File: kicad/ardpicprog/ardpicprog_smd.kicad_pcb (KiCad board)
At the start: 2 copper layers, 69.2 x 53.9 mm, 37 parts, among them P1 CONN_01X06, P2 CONN_01X02, Q1 BC548, SW1 SW_PUSH, U1 PIC16F627, U2 MC34063, U3 LM78L12ACZ

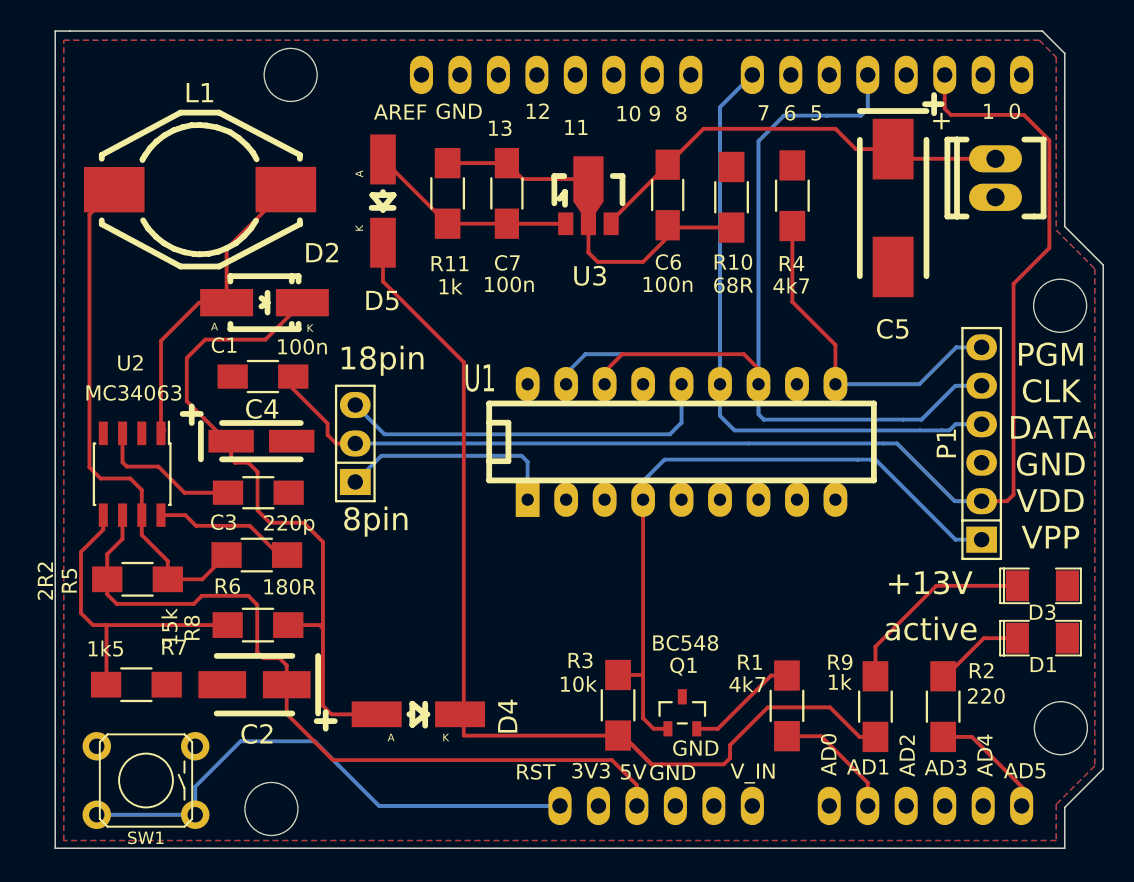
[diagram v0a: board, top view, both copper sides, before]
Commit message: to fcking much changes to commit it separatly, lets go with everything in one commit, git will love me for sure :D
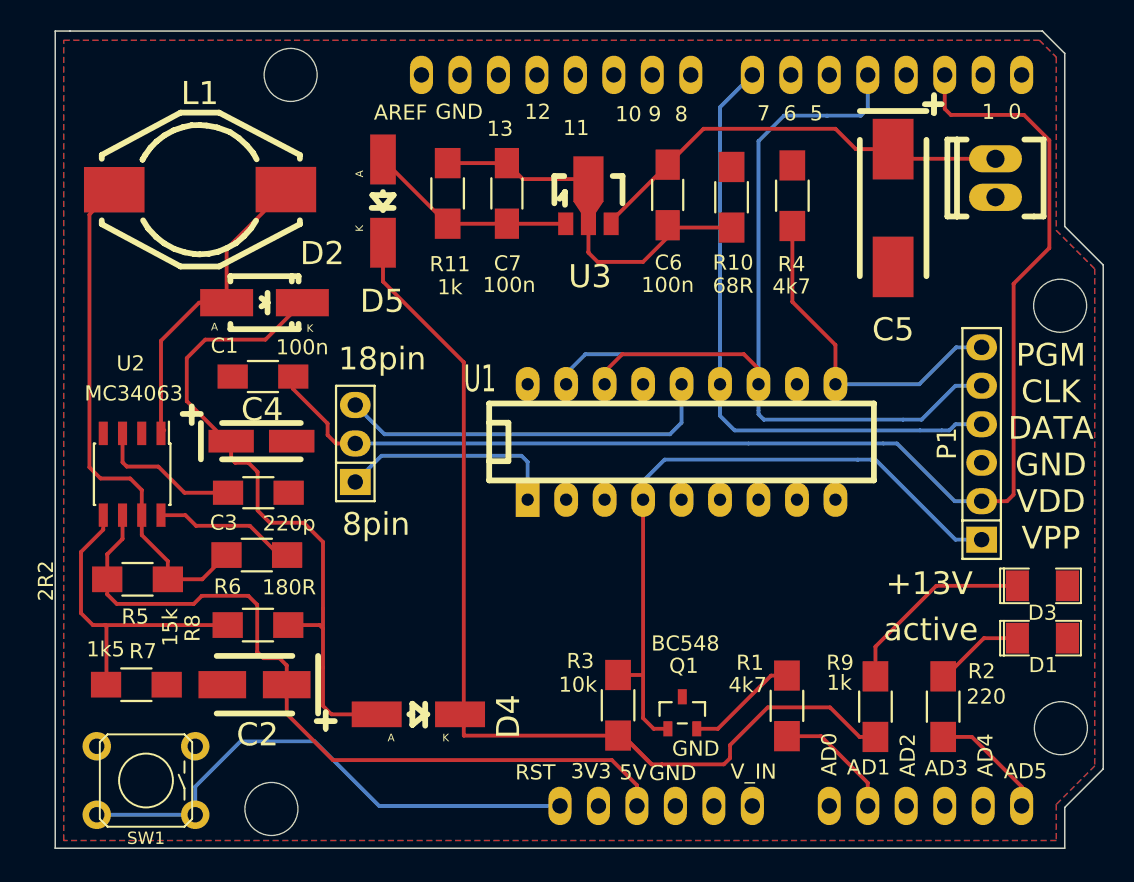
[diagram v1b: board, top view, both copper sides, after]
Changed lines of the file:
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@@
-(kicad_pcb (version 20160815) (host pcbnew 4.1.0-alpha+201608211231+7083~46~ubuntu16.04.1-product)
+(kicad_pcb (version 20171130) (host pcbnew 5.0.0-rc2-dev-unknown-ce1bd4c~62~ubuntu16.04.1)
   (general
-    (links 74)
-    (no_connects 1)
-    (area 129.286799 76.099199 198.576401 130.148801)
     (thickness 1.6)
     (drawings 34)
@@
     (pad_to_mask_clearance 0)
     (aux_axis_origin 0 0)
-    (visible_elements FFFFFF7F)
+    (visible_elements FFFDFF7F)
     (pcbplotparams
-      (layerselection 0x00030_80000001)
+      (layerselection 0x010fc_ffffffff)
       (usegerberextensions false)
+      (usegerberattributes false)
+      (usegerberadvancedattributes false)
+      (creategerberjobfile false)
       (excludeedgelayer true)
       (linewidth 0.100000)
@@
       (drillshape 0)
       (scaleselection 1)
-      (outputdirectory ""))
+      (outputdirectory /home/nail/src/hw/kicad/ardpicprog/prod/))
   )
   (net 0 "")
@@
     (uvia_dia 0.508)
     (uvia_drill 0.127)
-    (diff_pair_gap 0.25)
-    (diff_pair_width 0.2)
     (add_net 13V)
     (add_net 5V)
@@
     (attr smd)
     (fp_text reference C4 (at 0.0508 -2.0828 180) (layer F.SilkS)
-      (effects (font (thickness 0.3048)))
+      (effects (font (size 1.524 1.524) (thickness 0.3048)))
     )
     (fp_text value 10m/16V (at -0.09906 3.0988) (layer F.SilkS) hide
-      (effects (font (thickness 0.3048)))
+      (effects (font (size 1.524 1.524) (thickness 0.3048)))
     )
     (fp_text user + (at -4.59994 -1.80086) (layer F.SilkS)
-      (effects (font (thickness 0.3048)))
+      (effects (font (size 1.524 1.524) (thickness 0.3048)))
     )
     (fp_line (start -2.60096 1.19888) (end 2.60096 1.19888) (layer F.SilkS) (width 0.381))
@@
     (attr smd)
     (fp_text reference C5 (at 8.0264 0) (layer F.SilkS)
-      (effects (font (thickness 0.3048)))
+      (effects (font (size 1.524 1.524) (thickness 0.3048)))
     )
     (fp_text value 33m/35V (at -0.09906 3.59918 270) (layer F.SilkS) hide
-      (effects (font (thickness 0.3048)))
+      (effects (font (size 1.524 1.524) (thickness 0.3048)))
     )
     (fp_line (start -6.40334 -2.19964) (end -6.40334 2.19964) (layer F.SilkS) (width 0.381))
     (fp_line (start -4.50088 2.19964) (end 4.50088 2.19964) (layer F.SilkS) (width 0.381))
     (fp_line (start 4.50088 -2.19964) (end -4.50088 -2.19964) (layer F.SilkS) (width 0.381))
-    (fp_text user + (at -5.7404 -3.1496 270) (layer F.SilkS)
-      (effects (font (thickness 0.3048)))
+    (fp_text user + (at -6.8072 -2.54 270) (layer F.SilkS)
+      (effects (font (size 1.524 1.524) (thickness 0.3048)))
     )
     (fp_line (start -6.858 -3.20294) (end -6.858 -2.10312) (layer F.SilkS) (width 0.381))
@@
     (attr smd)
     (fp_text reference D2 (at 3.81 -3.2512) (layer F.SilkS)
-      (effects (font (thickness 0.3048)))
+      (effects (font (size 1.524 1.524) (thickness 0.3048)))
     )
     (fp_text value 1N5819 (at 0 3.81) (layer F.SilkS) hide
-      (effects (font (thickness 0.3048)))
+      (effects (font (size 1.524 1.524) (thickness 0.3048)))
     )
     (fp_line (start 0.20066 -0.65024) (end 0.20066 0.65024) (layer F.SilkS) (width 0.381))
@@
     (attr smd)
     (fp_text reference L1 (at 0 -6.35) (layer F.SilkS)
-      (effects (font (thickness 0.3048)))
+      (effects (font (size 1.524 1.524) (thickness 0.3048)))
     )
     (fp_text value 220uH (at 1.27 7.62) (layer F.SilkS) hide
-      (effects (font (thickness 0.3048)))
+      (effects (font (size 1.524 1.524) (thickness 0.3048)))
     )
     (fp_line (start 0 -0.254) (end 0 0.254) (layer F.Adhes) (width 0.381))
@@
     (tags "Socket, MOLEX, KK, RM 2.54mm, Lock, 2pin, straight,")
     (fp_text reference P2 (at 0 -4.445 90) (layer F.SilkS) hide
-      (effects (font (thickness 0.3048)))
+      (effects (font (size 1.524 1.524) (thickness 0.3048)))
     )
     (fp_text value CONN_01X02 (at -0.635 5.08 90) (layer F.SilkS) hide
-      (effects (font (thickness 0.3048)))
+      (effects (font (size 1.524 1.524) (thickness 0.3048)))
     )
     (fp_line (start -2.54 -2.54) (end 2.54 -2.54) (layer F.SilkS) (width 0.381))
@@
     (tags "resistor 1206")
     (attr smd)
-    (fp_text reference R5 (at -4.4704 0.1016 90) (layer F.SilkS)
+    (fp_text reference R5 (at -0.1524 2.4638 180) (layer F.SilkS)
       (effects (font (size 1 1) (thickness 0.15)))
     )
@@
     (tags "resistor 1206")
     (attr smd)
-    (fp_text reference R7 (at 2.4892 -2.4384) (layer F.SilkS)
+    (fp_text reference R7 (at 0.4318 -2.2098) (layer F.SilkS)
       (effects (font (size 1 1) (thickness 0.15)))
     )
@@
     (attr smd)
     (fp_text reference U3 (at 0.1016 5.334) (layer F.SilkS)
-      (effects (font (thickness 0.3048)))
+      (effects (font (size 1.524 1.524) (thickness 0.3048)))
     )
     (fp_text value LM78L12ACZ (at -0.20066 4.59994) (layer F.SilkS) hide
-      (effects (font (thickness 0.3048)))
+      (effects (font (size 1.524 1.524) (thickness 0.3048)))
     )
     (fp_line (start -1.89992 0.20066) (end -1.651 -0.09906) (layer F.SilkS) (width 0.381))
@@
     (at 129.6416 129.8448)
     (fp_text reference SHIELD1 (at 5.715 -57.15) (layer F.SilkS) hide
-      (effects (font (thickness 0.3048)))
+      (effects (font (size 1.524 1.524) (thickness 0.3048)))
     )
     (fp_text value ARDUINO_SHIELD (at 10.16 -54.61) (layer F.SilkS) hide
-      (effects (font (thickness 0.3048)))
+      (effects (font (size 1.524 1.524) (thickness 0.3048)))
     )
     (fp_circle (center 13.97 -2.54) (end 16.002 -1.524) (layer Dwgs.User) (width 0.381))
@@
     (attr smd)
     (fp_text reference D4 (at 5.9436 0.1524 -270) (layer F.SilkS)
-      (effects (font (thickness 0.3048)))
+      (effects (font (size 1.524 1.524) (thickness 0.3048)))
     )
     (fp_text value DIODE (at 0 3.81) (layer F.SilkS) hide
-      (effects (font (thickness 0.3048)))
+      (effects (font (size 1.524 1.524) (thickness 0.3048)))
     )
     (fp_line (start 0.44958 0) (end 0.59944 0) (layer F.SilkS) (width 0.381))
@@
     (attr smd)
     (fp_text reference D5 (at 6.604 0.0508) (layer F.SilkS)
-      (effects (font (thickness 0.3048)))
+      (effects (font (size 1.524 1.524) (thickness 0.3048)))
     )
     (fp_text value DIODE (at 0 3.81 270) (layer F.SilkS) hide
-      (effects (font (thickness 0.3048)))
+      (effects (font (size 1.524 1.524) (thickness 0.3048)))
     )
     (fp_line (start 0.44958 0) (end 0.59944 0) (layer F.SilkS) (width 0.381))
@@
     (tags "Mounting hole, Befestigungsbohrung, 3,5mm, No Annular, Kein Restring,")
     (fp_text reference MH (at 0 -4.50088) (layer F.SilkS) hide
-      (effects (font (thickness 0.3048)))
+      (effects (font (size 1.524 1.524) (thickness 0.3048)))
     )
     (fp_text value MountingHole_3-5mm_RevA_Date21Jun2010 (at 0 5.00126) (layer F.SilkS) hide
-      (effects (font (thickness 0.3048)))
+      (effects (font (size 1.524 1.524) (thickness 0.3048)))
     )
     (fp_circle (center 0 0) (end 3.50012 0) (layer Cmts.User) (width 0.381))
@@
     (tags "Mounting hole, Befestigungsbohrung, 3,5mm, No Annular, Kein Restring,")
     (fp_text reference MH (at 0 -4.50088) (layer F.SilkS) hide
-      (effects (font (thickness 0.3048)))
+      (effects (font (size 1.524 1.524) (thickness 0.3048)))
     )
     (fp_text value MountingHole_3-5mm_RevA_Date21Jun2010 (at 0 5.00126) (layer F.SilkS) hide
-      (effects (font (thickness 0.3048)))
+      (effects (font (size 1.524 1.524) (thickness 0.3048)))
     )
     (fp_circle (center 0 0) (end 3.50012 0) (layer Cmts.User) (width 0.381))
@@
     (tags "Mounting hole, Befestigungsbohrung, 3,5mm, No Annular, Kein Restring,")
     (fp_text reference MH (at 0 -4.50088) (layer F.SilkS) hide
-      (effects (font (thickness 0.3048)))
+      (effects (font (size 1.524 1.524) (thickness 0.3048)))
     )
     (fp_text value MountingHole_3-5mm_RevA_Date21Jun2010 (at 0 5.00126) (layer F.SilkS) hide
-      (effects (font (thickness 0.3048)))
+      (effects (font (size 1.524 1.524) (thickness 0.3048)))
     )
     (fp_circle (center 0 0) (end 3.50012 0) (layer Cmts.User) (width 0.381))
@@
     (tags "Mounting hole, Befestigungsbohrung, 3,5mm, No Annular, Kein Restring,")
     (fp_text reference MH (at 0 -4.50088) (layer F.SilkS) hide
-      (effects (font (thickness 0.3048)))
+      (effects (font (size 1.524 1.524) (thickness 0.3048)))
     )
     (fp_text value MountingHole_3-5mm_RevA_Date21Jun2010 (at 0 5.00126) (layer F.SilkS) hide
-      (effects (font (thickness 0.3048)))
+      (effects (font (size 1.524 1.524) (thickness 0.3048)))
     )
     (fp_circle (center 0 0) (end 3.50012 0) (layer Cmts.User) (width 0.381))
@@
     (attr smd)
     (fp_text reference C2 (at -0.20066 -3.29946 180) (layer F.SilkS)
-      (effects (font (thickness 0.3048)))
+      (effects (font (size 1.524 1.524) (thickness 0.3048)))
     )
     (fp_text value 10m/6,3V (at -0.09906 3.59918 180) (layer F.SilkS) hide
-      (effects (font (thickness 0.3048)))
+      (effects (font (size 1.524 1.524) (thickness 0.3048)))
     )
     (fp_text user + (at -4.70154 -2.4003 180) (layer F.SilkS)
-      (effects (font (thickness 0.3048)))
+      (effects (font (size 1.524 1.524) (thickness 0.3048)))
     )
     (fp_line (start -4.20116 -1.89992) (end -4.20116 1.89992) (layer F.SilkS) (width 0.381))
@@
     (effects (font (size 1.5 1.5) (thickness 0.3)))
   )
-  (gr_text 8pin (at 150.5204 108.4072) (layer F.SilkS)
+  (gr_text 8pin (at 150.5204 108.712) (layer F.SilkS)
     (effects (font (size 1.5 1.5) (thickness 0.3)))
   )
